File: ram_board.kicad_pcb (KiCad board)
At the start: 4 copper layers, 72.6 x 31.6 mm, 25 parts, among them J1 Bus, J2 PWR, SW1 Config, U1 IS61LV5128AL-10TLI, U2 SST39VF040-70-4C-NHE, U3 74LVC2G240, U4 74LVC2G240

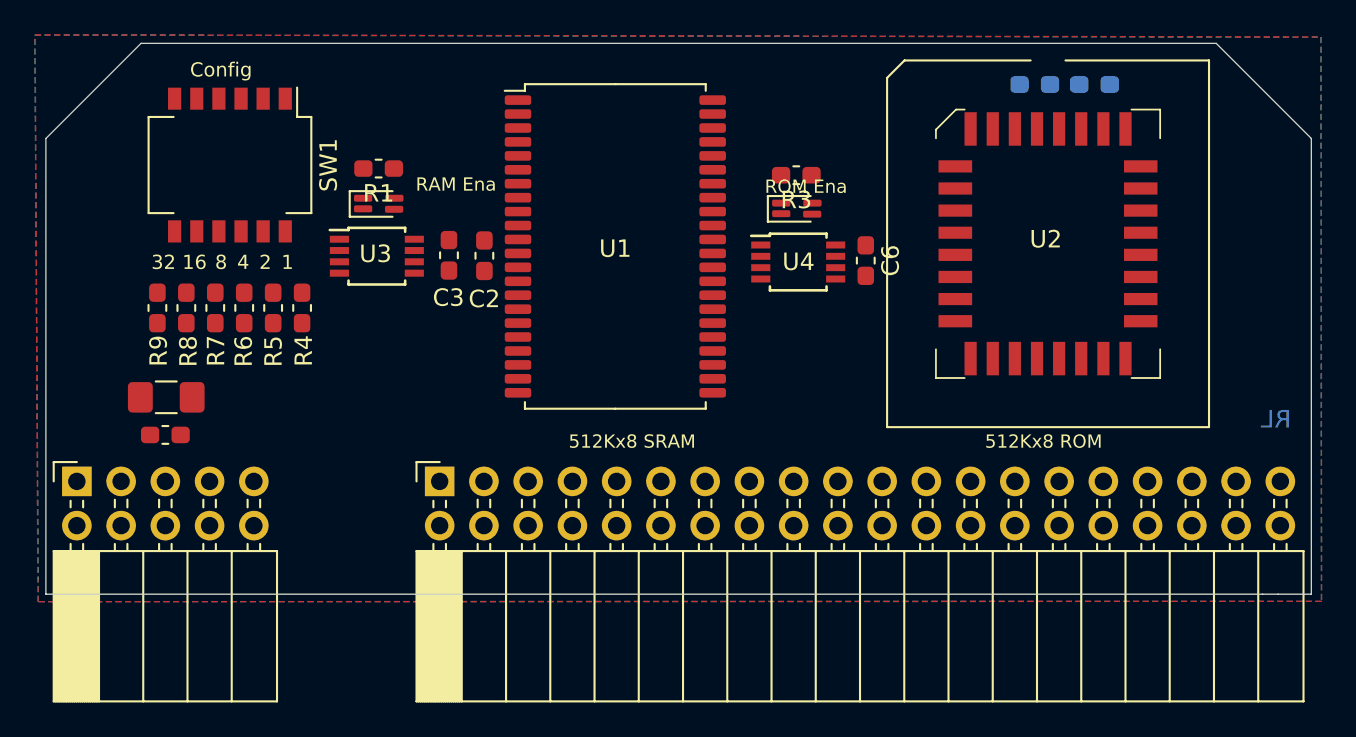
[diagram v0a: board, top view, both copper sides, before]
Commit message: simplified pins, finished routing
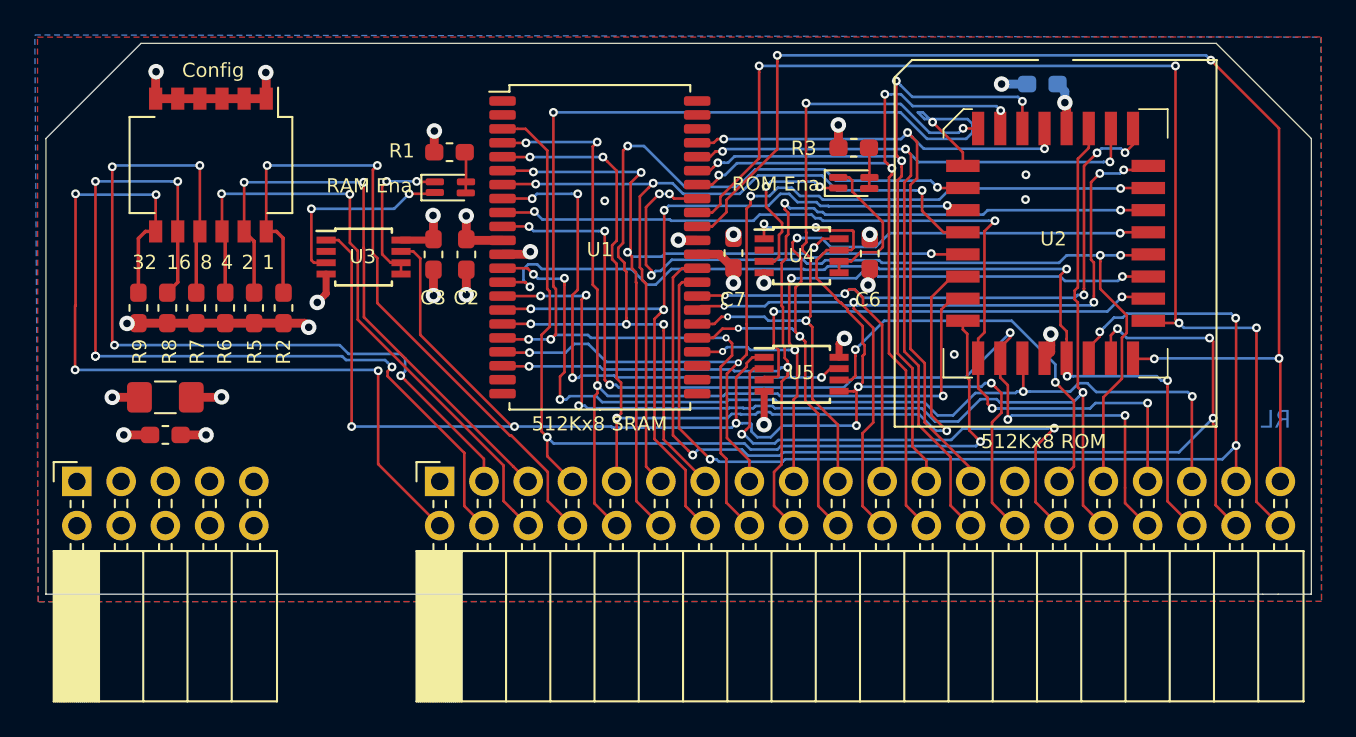
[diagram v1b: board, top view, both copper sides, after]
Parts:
- removed R4: 10K, Resistor_SMD:R_0603_1608Metric_Pad1.05x0.95mm_HandSolder
- added C7: 100nF, Capacitor_SMD:C_0603_1608Metric_Pad1.05x0.95mm_HandSolder, F.Cu at (156.9, 84.6)
- added U5: 74LVC2G32, Package_SO:TSSOP-8_3x3mm_P0.65mm, F.Cu at (160.9, 91.5)
- R2: moved to F.Cu
- moved R2 48.3 mm to (131.1, 87.7), turned to 270 degrees
- moved D2 4.22 mm to (140.7, 80.8)
- moved R1 4.18 mm to (140.6, 78.8)
- moved R3 3.65 mm to (163.8, 78.5)
- moved D3 3.59 mm to (163.8, 80.5)
- moved R5 1.09 mm to (129.4, 87.7)
- moved R6 1.09 mm to (127.8, 87.7)
- moved R7 1.09 mm to (126.1, 87.7)
- moved SW1 1.09 mm to (126.9, 79.5)
- moved R8 1.09 mm to (124.4, 87.7)
- moved R9 1.09 mm to (122.8, 87.7)
- moved C2 1.04 mm to (141.6, 84.6)
- moved U1 0.89 mm to (149.3, 84.2)
- moved C3 0.89 mm to (139.7, 84.6)
- moved U3 0.76 mm to (135.7, 84.8)
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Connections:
- J1 pad 11: /A2 -> /A4
- J1 pad 13: /A4 -> /A6
- J1 pad 2: /SW1_3 -> /SW1_5
- J1 pad 27: /RAM_OE -> (no net)
- J1 pad 28: /RAM_CE -> /~ENA
- J1 pad 29: /D0 -> /~ROM
- J1 pad 3: /SW1_5 -> /SW1_3
- J1 pad 30: /RAM_WE -> /~RAM
- J1 pad 31: /D2 -> /~RD
- J1 pad 32: /D1 -> /~WR
- J1 pad 33: /D4 -> /D0
- J1 pad 34: /D3 -> /D1
- J1 pad 35: /D6 -> /D2
- J1 pad 36: /D5 -> /D3
- J1 pad 37: /ROM_CE -> /D4
- J1 pad 38: /D7 -> /D5
- J1 pad 39: /ROM_WE -> /D6
- J1 pad 4: /SW1_2 -> /SW1_4
- J1 pad 40: /ROM_OE -> /D7
- J1 pad 5: /SW1_4 -> /SW1_1
- J1 pad 6: /SW1_1 -> /SW1_2
- J1 pad 7: (no net) -> /A0
- J1 pad 9: /A0 -> /A2
- R2 pad 1: /ROM_WE -> /SW1_0
- U1 pad 15: /RAM_WE -> /~WR
- U1 pad 37: /RAM_OE -> /~RD
- U1 pad 8: /RAM_CE -> Net-(U1-Pad8)
- U2 pad 22: /ROM_CE -> Net-(U2-Pad22)
- U2 pad 24: /ROM_OE -> /~RD
- U2 pad 31: /ROM_WE -> /~WR
- U3 pad 2: /RAM_CE -> (no net)
- U4 pad 2: /ROM_CE -> (no net)
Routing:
- net /~ENA: track 0.00 -> 98.3 mm, vias 0 -> 8
- net /D6: track 0.00 -> 71.5 mm, vias 0 -> 4
- net /A7: track 0.00 -> 71.2 mm, vias 0 -> 5
- net /D7: track 0.00 -> 67.5 mm, vias 0 -> 4
- net /~WR: track 0.00 -> 65.5 mm, vias 0 -> 4
- net /D5: track 0.00 -> 62.1 mm, vias 0 -> 4
- net /D4: track 0.00 -> 62.0 mm, vias 0 -> 4
- net /D1: track 0.00 -> 58.4 mm, vias 0 -> 6
- net /A9: track 0.00 -> 57.5 mm, vias 0 -> 4
- net /D3: track 0.00 -> 56.4 mm, vias 0 -> 4
- net /D2: track 0.00 -> 55.8 mm, vias 0 -> 5
- net /A0: track 0.00 -> 55.8 mm, vias 0 -> 2
- net /A8: track 0.00 -> 55.3 mm, vias 0 -> 4
- net /A1: track 0.00 -> 55.2 mm, vias 0 -> 4
- net /A2: track 0.00 -> 55.0 mm, vias 0 -> 4
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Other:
- rule via_min_drill: 0.254 -> 0.2032
- rule via_min_size: 0.508 -> 0.4064
